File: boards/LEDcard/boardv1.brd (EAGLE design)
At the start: 103.8 x 71.1 mm, 38 parts, among them K1 NA, K2 NA, K3 NA, K4 NA, K5 NA, K6 NA, X1 112404, X2 112404, X3 112404, X4 112404, X5 112404, X6 112404, X7 112404, X8 112404

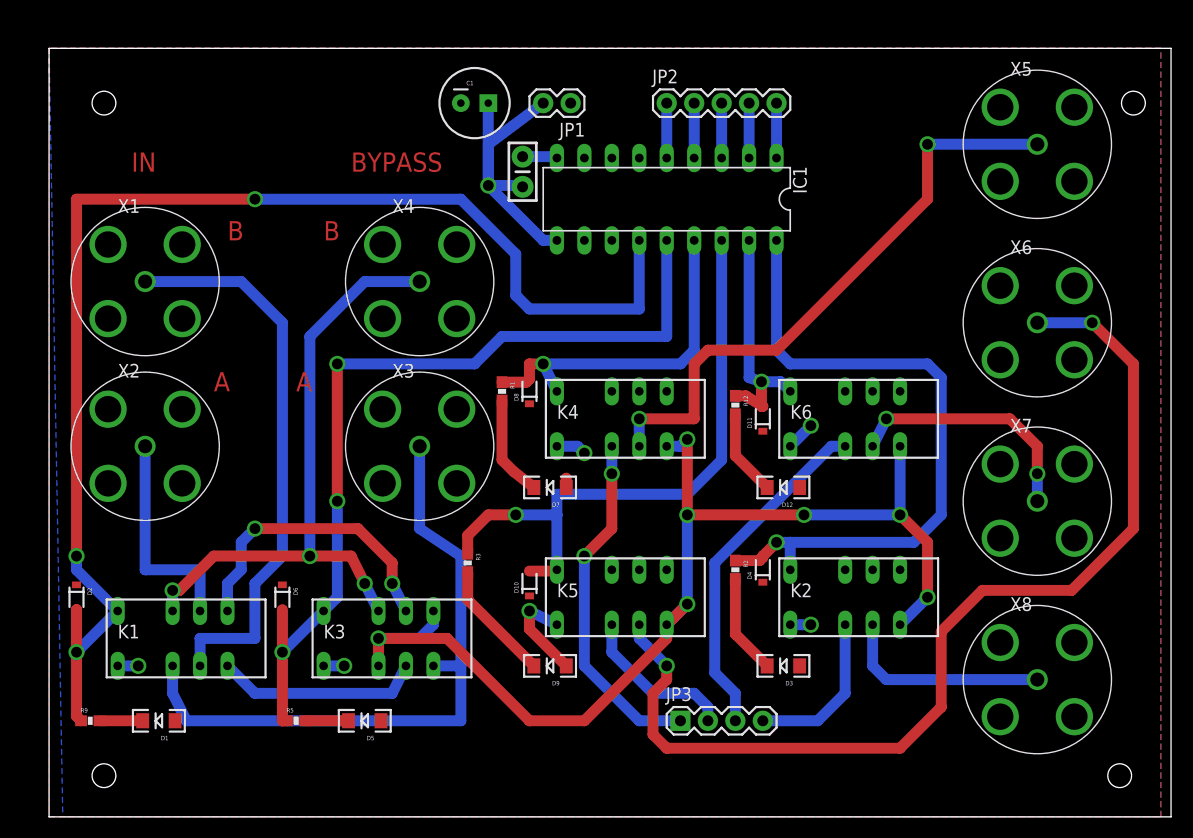
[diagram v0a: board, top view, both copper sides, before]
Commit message: Board update
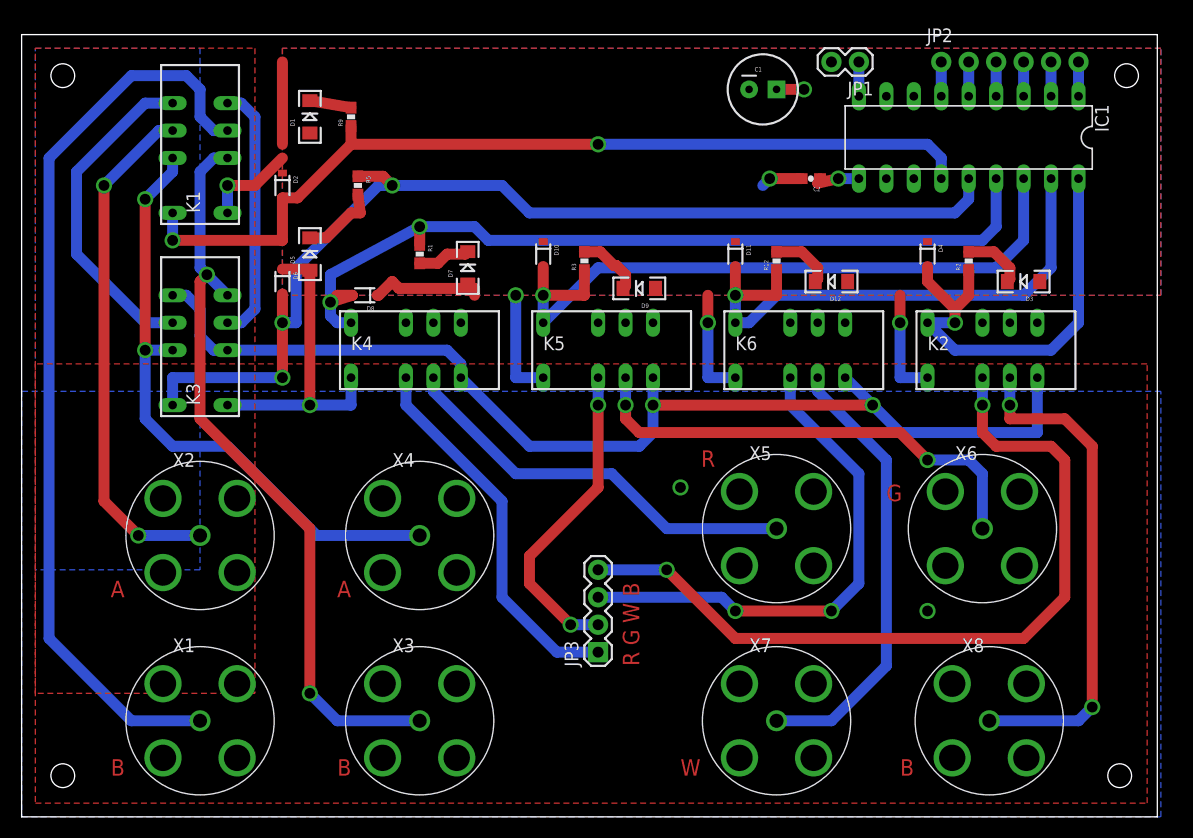
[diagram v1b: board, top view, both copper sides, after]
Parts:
- C2: device SparkFun-Capacitors:CAP-PTH-SMALL-KIT -> SparkFun-Capacitors:0603-CAP
- JP2: device SparkFun-Connectors:1X05 -> SparkFun-Connectors:1X06_NO_SILK_YES_STOP
- moved R9 60.9 mm to (27.9, 61.0), turned to 90 degrees
- moved D1 57.6 mm to (24.1, 61.0), turned to 90 degrees
- moved R5 49.9 mm to (28.6, 54.6), turned to 270 degrees
- moved K1 45.7 mm to (14.0, 58.4), turned to 90 degrees
- moved D5 43.5 mm to (24.1, 48.3), turned to 90 degrees
- moved X5 43.0 mm to (67.3, 22.9)
- moved D2 42.6 mm to (21.6, 54.6)
- moved D3 41.9 mm to (90.2, 45.7)
- moved X1 41.0 mm to (14.0, 5.08)
- moved D9 35.9 mm to (54.6, 45.1)
- moved R2 35.8 mm to (85.1, 47.6), turned to 90 degrees
- moved K3 33.1 mm to (14.0, 40.6), turned to 90 degrees
- moved D4 32.9 mm to (81.3, 48.3), turned to 270 degrees
- moved X7 31.5 mm to (67.3, 5.08)
- moved D10 30.5 mm to (45.7, 48.3), turned to 270 degrees
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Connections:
- removed net N$21: IC1.1, JP2.5
- removed net N$22: IC1.2, JP2.4
- removed net N$23: IC1.3, JP2.3
- new net GND2: C1.2, C2.2, IC1.9, JP1.1
- new net N$10: IC1.2, JP2.5
- new net N$11: IC1.3, JP2.4
- new net N$8: IC1.6, JP2.1
- new net N$9: IC1.1, JP2.6
- net GND: no longer C1.2, C2.2, IC1.9, JP1.1
- net N$24: now also JP2.3; no longer JP2.2
- net N$25: now also JP2.2; no longer JP2.1
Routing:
- net ARDUINO1: track 15.0 -> 73.8 mm, vias 0 -> 2
- net OUTPUT2: track 94.9 -> 44.0 mm
- net R4: track 32.8 -> 80.3 mm, vias 1 -> 2
- net VCC: track 50.8 -> 94.0 mm
- net R6: track 124.3 -> 83.8 mm, vias 3 -> 2
- net INPUTA: track 52.2 -> 84.8 mm
- net R2: track 22.2 -> 50.9 mm
- net INPUTB: track 20.3 -> 47.9 mm, vias 0 -> 2
- net OUTPUT4: track 19.6 -> 46.7 mm, vias 0 -> 2
- net R1: track 62.6 -> 42.3 mm
- net R5: track 79.9 -> 99.8 mm
- net OUTPUT3: track 22.9 -> 41.6 mm, vias 2 -> 0
- net OUTPUT1: track 55.8 -> 38.3 mm, vias 2 -> 0
- net ARDUINO2: track 31.9 -> 47.4 mm, vias 0 -> 2
- net ARDUINO3: track 14.8 -> 29.6 mm, vias 0 -> 2
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- added copper zone on layer 1, net GND
- added copper zone on layer 16, net GND2
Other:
- board size 103.8 x 71.1 mm -> 105.1 x 72.4 mm
- board text added: "G"
- board text added: "R"
- board text added: "R G W B"
- board text added: "W"
- board text removed: "BYPASS"
- board text removed: "IN"
